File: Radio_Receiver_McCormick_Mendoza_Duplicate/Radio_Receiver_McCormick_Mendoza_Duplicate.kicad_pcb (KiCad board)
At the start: 4 copper layers, 100 x 100 mm, 243 parts, among them J1 VBAT, J10 CLK_2, J11 I_LO, J12 Q_LO, J13 I_0, J14 I_180, J15 Q_90, J16 Q_270, J17 I_RAW, J18 Conn_01x02_Female, J19 Conn_01x02_Female, J2 GND, J20 Q_RAW, J21 SDR Out, J23 VDDA, J24 CLK_0, J25 OLED, J26 +5V, J3 3.3VA, J33 XFIL_IN, J34 XFIL_OUT, J35 3.5mm_Jack, J36 +5RAW, J37 4.5V, J38 DAC_FLT, J39 VDD, J4 4.5VA, J40 DAC_FMT, J41 V_DIV, J42 VDDA/2, J45 CENTER_TAP, J46 3.5mm_Jack, J47 FIL_IN, J5 Conn_Coaxial, J6 Conn_01x02, J7 Micro_SD-TF_PUSH, J8 FIL_OUT, J9 CLK_1, SW1 RotaryEncoder_Switch_MP, SW6 09.03290.01, T1 Transformer_1P_SS, U1 TPS7A2045PDQN, U10 OPA1612AID, U11 INA821ID, U12 PCM1808PWR, U13 SN74CBT3253CDBR, U14 PCM5102A, U2 TPS7A2045PDQN, U3 TPS72733DSER, U4 Pico, U5 Si5351A-B-GT, U6 SN74AC74DR, U8 SN74CBT3253CDBR, U9 INA821ID, Y1 ASTX-H11-24.576MHZ-T

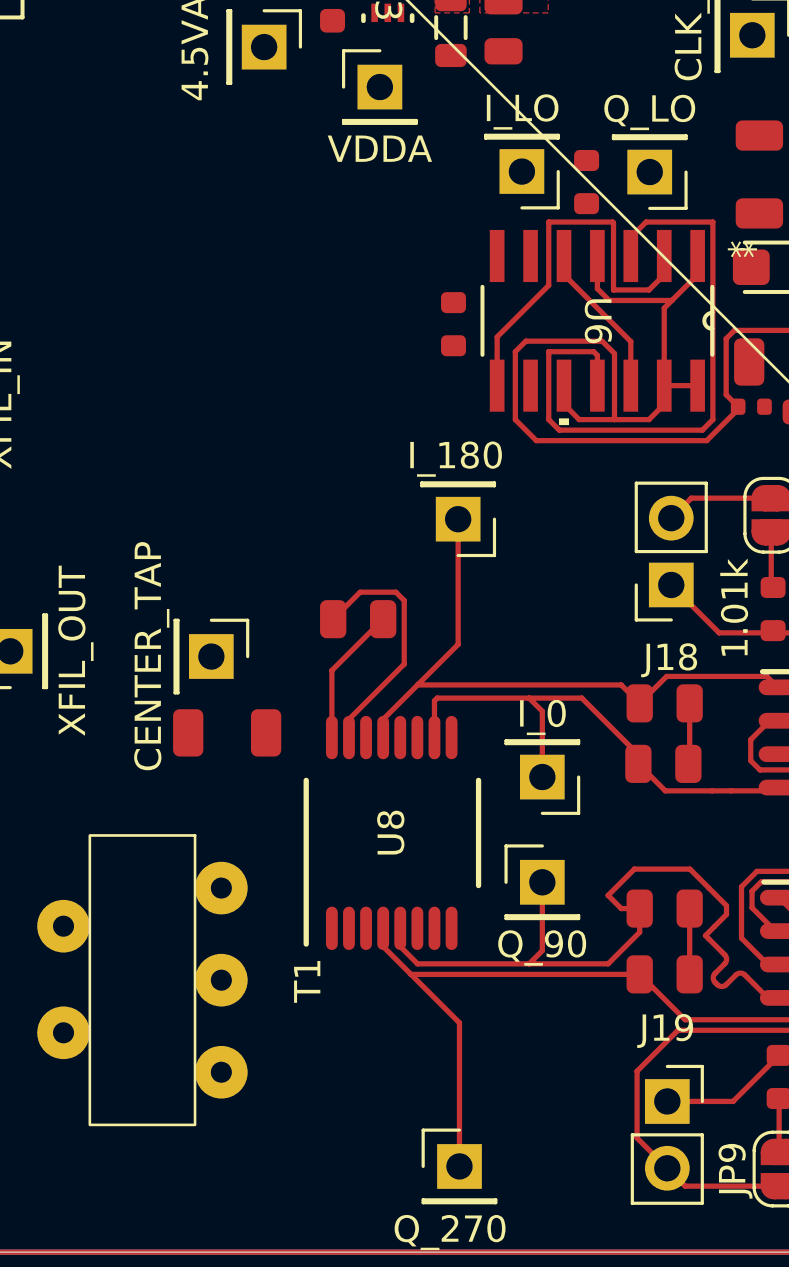
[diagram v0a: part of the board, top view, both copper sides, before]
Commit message: tracing more things
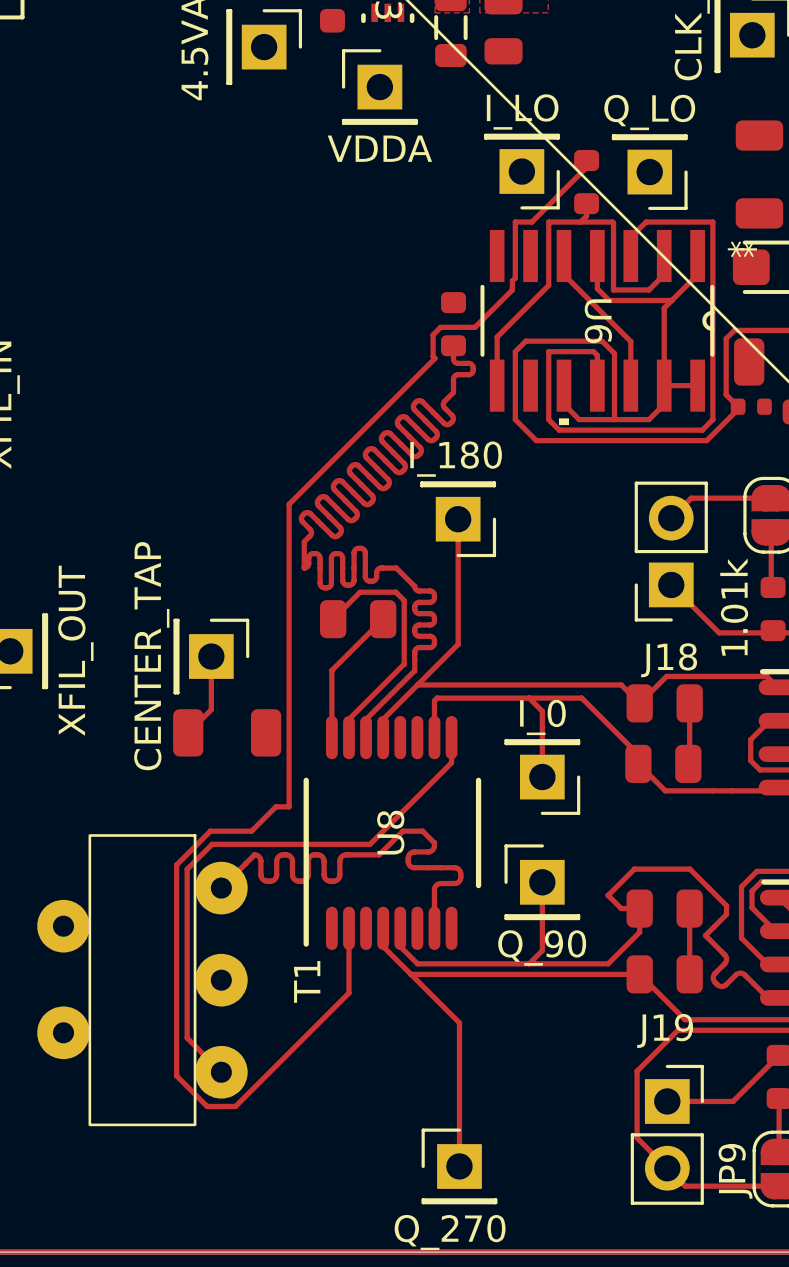
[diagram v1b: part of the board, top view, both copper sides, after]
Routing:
- net /Clock Generator/Q_LO: track 0.00 -> 54.9 mm
- net /Clock Generator/I_LO: track 0.00 -> 54.1 mm
- net /RF_IN2: track 0.00 -> 20.9 mm
- net /RF_IN1: track 0.00 -> 20.4 mm
- net /ADC-24bit/VDDA/2: track 14.8 -> 18.1 mm
- net Net-(J12-Pin_1): track 14.9 -> 15.7 mm
